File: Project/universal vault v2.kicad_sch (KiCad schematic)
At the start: 213 parts, among them J1 USB_C_Receptacle_USB2.0, SW1 RotaryEncoder_Switch, SW2 RotaryEncoder_Switch, SW3 RotaryEncoder_Switch, SW4 SKQGABE010, SW5 RotaryEncoder_Switch, U1 STM32F072CBUx, U2 XC6206PxxxMR, U5 74AHCT1G125

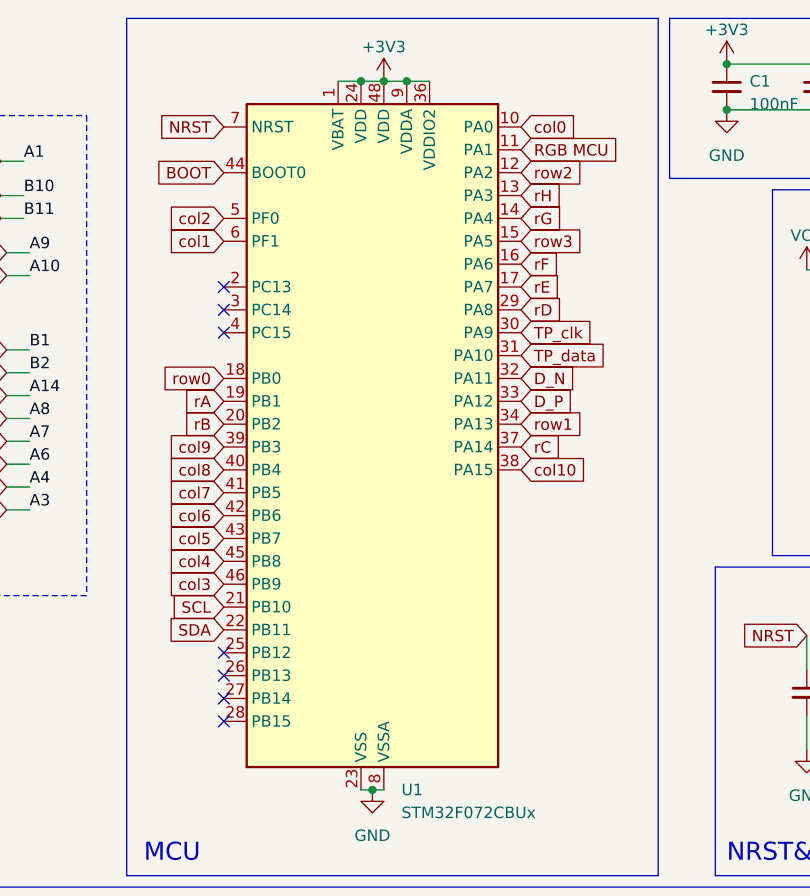
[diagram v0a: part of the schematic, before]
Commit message: changed rgb pin for better software hardware compatibility & fresh production files
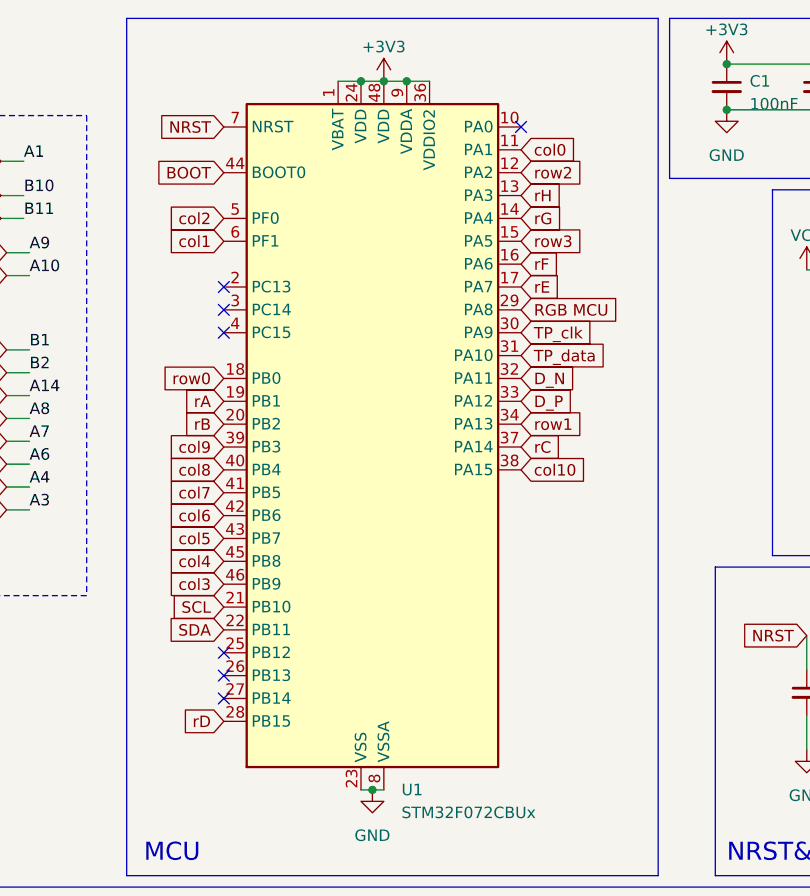
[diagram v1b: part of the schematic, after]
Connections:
- net RGB MCU: now also U1.29 (PA8); no longer U1.11 (PA1)
- net col0: now also U1.11 (PA1); no longer U1.10 (PA0)
- net rD: now also U1.28 (PB15); no longer U1.29 (PA8)
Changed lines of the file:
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@@
   (no_connect (at 70.485 85.725))
   (no_connect (at 217.805 74.93))
-  (no_connect (at 70.485 90.805))
   (no_connect (at 70.485 47.625))
+  (no_connect (at 103.505 24.765))
   (no_connect (at 70.485 88.265))
   (no_connect (at 70.485 83.185))
@@
     )
   )
-  (global_label "col0" (shape input) (at 103.505 24.765 0) (fields_autoplaced)
-    (effects (font (size 1.27 1.27)) (justify left))
-    (property "Intersheetrefs" "${INTERSHEET_REFS}" (at 110.5231 24.765 0)
+  (global_label "col0" (shape input) (at 103.505 27.305 0) (fields_autoplaced)
+    (effects (font (size 1.27 1.27)) (justify left))
+    (property "Intersheetrefs" "${INTERSHEET_REFS}" (at 110.5231 27.305 0)
       (effects (font (size 1.27 1.27)) (justify left) hide)
     )
@@
     )
   )
-  (global_label "rD" (shape input) (at 103.505 45.085 0) (fields_autoplaced)
-    (effects (font (size 1.27 1.27)) (justify left))
-    (property "Intersheetrefs" "${INTERSHEET_REFS}" (at 108.467 45.085 0)
-      (effects (font (size 1.27 1.27)) (justify left) hide)
+  (global_label "rD" (shape input) (at 70.485 90.805 180) (fields_autoplaced)
+    (effects (font (size 1.27 1.27)) (justify right))
+    (property "Intersheetrefs" "${INTERSHEET_REFS}" (at 65.523 90.805 0)
+      (effects (font (size 1.27 1.27)) (justify right) hide)
     )
   )
@@
     )
   )
-  (global_label "RGB MCU" (shape input) (at 103.505 27.305 0) (fields_autoplaced)
-    (effects (font (size 1.27 1.27)) (justify left))
-    (property "Intersheetrefs" "${INTERSHEET_REFS}" (at 115.0347 27.305 0)
-      (effects (font (size 1.27 1.27)) (justify left) hide)
-    )
+  (global_label "RGB MCU" (shape input) (at 103.505 45.085 0) (fields_autoplaced)
+    (effects (font (size 1.27 1.27)) (justify left))
+    (property "Intersheetrefs" "${INTERSHEET_REFS}" (at 115.0347 45.085 0)
+      (effects (font (size 1.27 1.27)) (justify left) hide)
+    )

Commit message: Revert "changed rgb pin for better software hardware compatibility & fresh production files"
This reverts commit 76bec49334091c1669f5db898bd2653646399791.
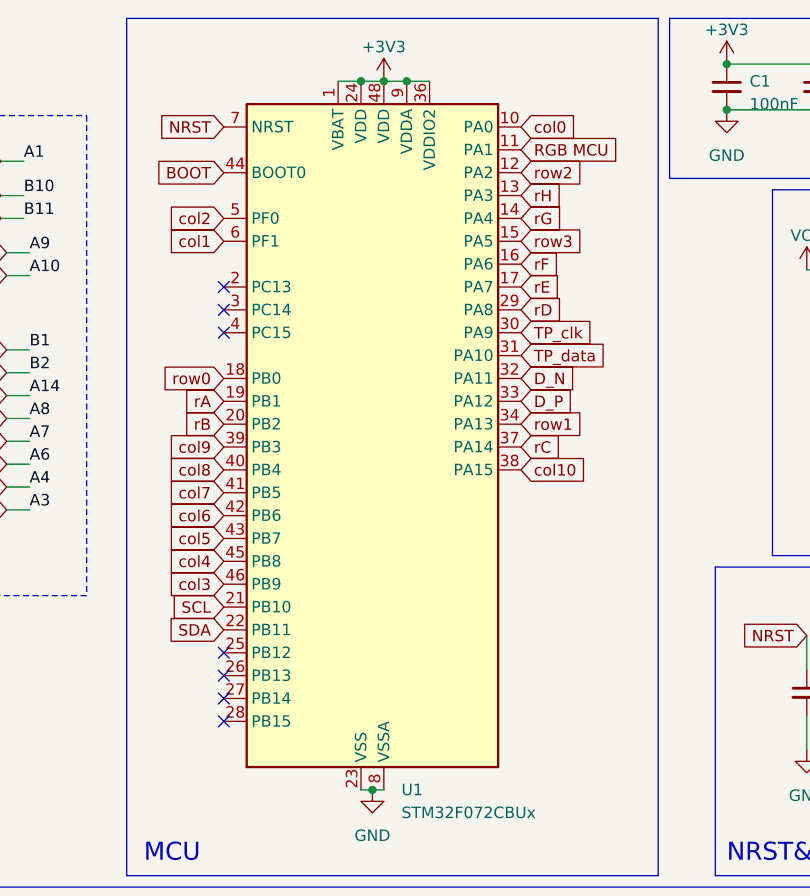
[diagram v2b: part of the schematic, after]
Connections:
- net RGB MCU: now also U1.11 (PA1); no longer U1.29 (PA8)
- net col0: now also U1.10 (PA0); no longer U1.11 (PA1)
- net rD: now also U1.29 (PA8); no longer U1.28 (PB15)
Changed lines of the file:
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@@
   (no_connect (at 70.485 85.725))
   (no_connect (at 217.805 74.93))
+  (no_connect (at 70.485 90.805))
   (no_connect (at 70.485 47.625))
-  (no_connect (at 103.505 24.765))
   (no_connect (at 70.485 88.265))
   (no_connect (at 70.485 83.185))
@@
     )
   )
-  (global_label "col0" (shape input) (at 103.505 27.305 0) (fields_autoplaced)
-    (effects (font (size 1.27 1.27)) (justify left))
-    (property "Intersheetrefs" "${INTERSHEET_REFS}" (at 110.5231 27.305 0)
+  (global_label "col0" (shape input) (at 103.505 24.765 0) (fields_autoplaced)
+    (effects (font (size 1.27 1.27)) (justify left))
+    (property "Intersheetrefs" "${INTERSHEET_REFS}" (at 110.5231 24.765 0)
       (effects (font (size 1.27 1.27)) (justify left) hide)
     )
@@
     )
   )
-  (global_label "rD" (shape input) (at 70.485 90.805 180) (fields_autoplaced)
-    (effects (font (size 1.27 1.27)) (justify right))
-    (property "Intersheetrefs" "${INTERSHEET_REFS}" (at 65.523 90.805 0)
-      (effects (font (size 1.27 1.27)) (justify right) hide)
+  (global_label "rD" (shape input) (at 103.505 45.085 0) (fields_autoplaced)
+    (effects (font (size 1.27 1.27)) (justify left))
+    (property "Intersheetrefs" "${INTERSHEET_REFS}" (at 108.467 45.085 0)
+      (effects (font (size 1.27 1.27)) (justify left) hide)
     )
   )
@@
     )
   )
-  (global_label "RGB MCU" (shape input) (at 103.505 45.085 0) (fields_autoplaced)
-    (effects (font (size 1.27 1.27)) (justify left))
-    (property "Intersheetrefs" "${INTERSHEET_REFS}" (at 115.0347 45.085 0)
-      (effects (font (size 1.27 1.27)) (justify left) hide)
-    )
+  (global_label "RGB MCU" (shape input) (at 103.505 27.305 0) (fields_autoplaced)
+    (effects (font (size 1.27 1.27)) (justify left))
+    (property "Intersheetrefs" "${INTERSHEET_REFS}" (at 115.0347 27.305 0)
+      (effects (font (size 1.27 1.27)) (justify left) hide)
+    )
